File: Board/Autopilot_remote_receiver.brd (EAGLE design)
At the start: 57.5 x 58.7 mm, 21 parts

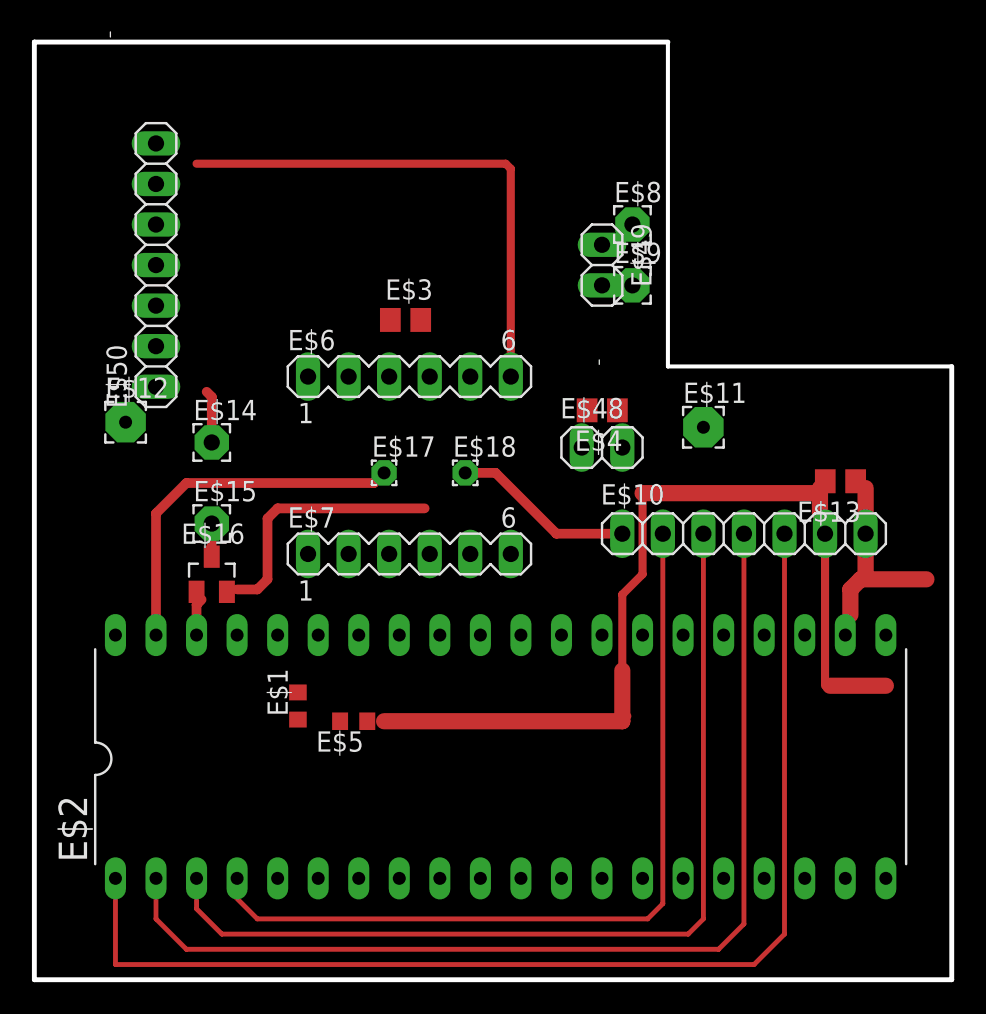
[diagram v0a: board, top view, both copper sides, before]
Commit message: Add schematic Update board
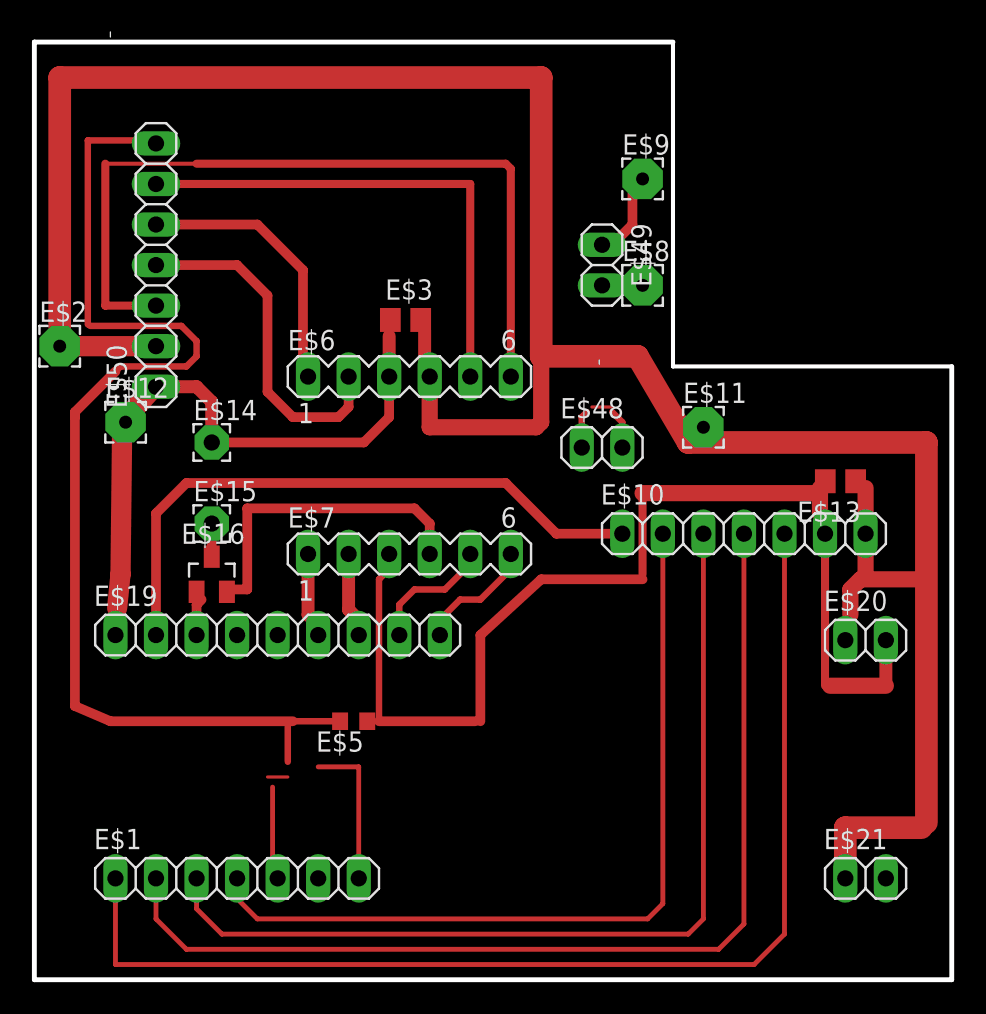
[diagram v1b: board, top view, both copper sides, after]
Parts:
- removed E$17, E$18: (no value), wirepad:1,6/0,8
- removed E$4: (no value), smd-ipc:C0805
- added E$19: (no value), pinhead:1X09
- added E$20, E$21: (no value), pinhead:1X02
- E$1: device smd-ipc:R0603 -> pinhead:1X07
- E$2: device ref-packages-longpad:DIL40 -> wirepad:2,54/0,8
- E$8, E$9: device wirepad:2,15/1,0 -> wirepad:2,54/0,8
- moved E$2 37.7 mm to (3.81, 40.3)
- moved E$1 11.4 mm to (14.9, 6.99), turned to 0 degrees
- moved E$9 6.70 mm to (40.3, 50.8)
- moved E$8 3.86 mm to (40.3, 44.1)
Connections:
- removed net S$10: E$2.1
- removed net S$5: E$14.1
- removed net S$8: E$17.1
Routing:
- net S$21: track 0.00 -> 35.9 mm
- net S$25: track 0.00 -> 30.2 mm
- net S$72: track 0.00 -> 23.8 mm
- net S$39: track 0.00 -> 19.8 mm
- net S$33: track 0.00 -> 18.4 mm
- net S$26: track 0.00 -> 17.5 mm
- net S$23: track 0.00 -> 16.5 mm
- net S$8: track 22.0 -> 37.3 mm
- net S$36: track 0.00 -> 15.0 mm
- net S$73: track 0.00 -> 14.9 mm
- net S$46: track 0.00 -> 12.4 mm
- net S$27: track 0.00 -> 11.7 mm
- net S$29: track 0.00 -> 11.5 mm
- net S$18: track 17.5 -> 6.00 mm
- net S$56: track 0.00 -> 11.4 mm
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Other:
- outline, holes or cut-outs redrawn
- board text added: "C1"
- board text added: "C2"
- board text added: "FET"
- board text added: "LogLevConv"
- board text added: "Maple mini"
- board text added: "RX480"
- board text added: "VT"
